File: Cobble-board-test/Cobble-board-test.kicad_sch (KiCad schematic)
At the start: 16 parts, among them J2 JST PH2.0 Battery, J3 Stemma PH, J4 Grove, Q1 SI2302DS, SW1 SW_Push, SW3 SW_VIBE, SW4 MSK22D27

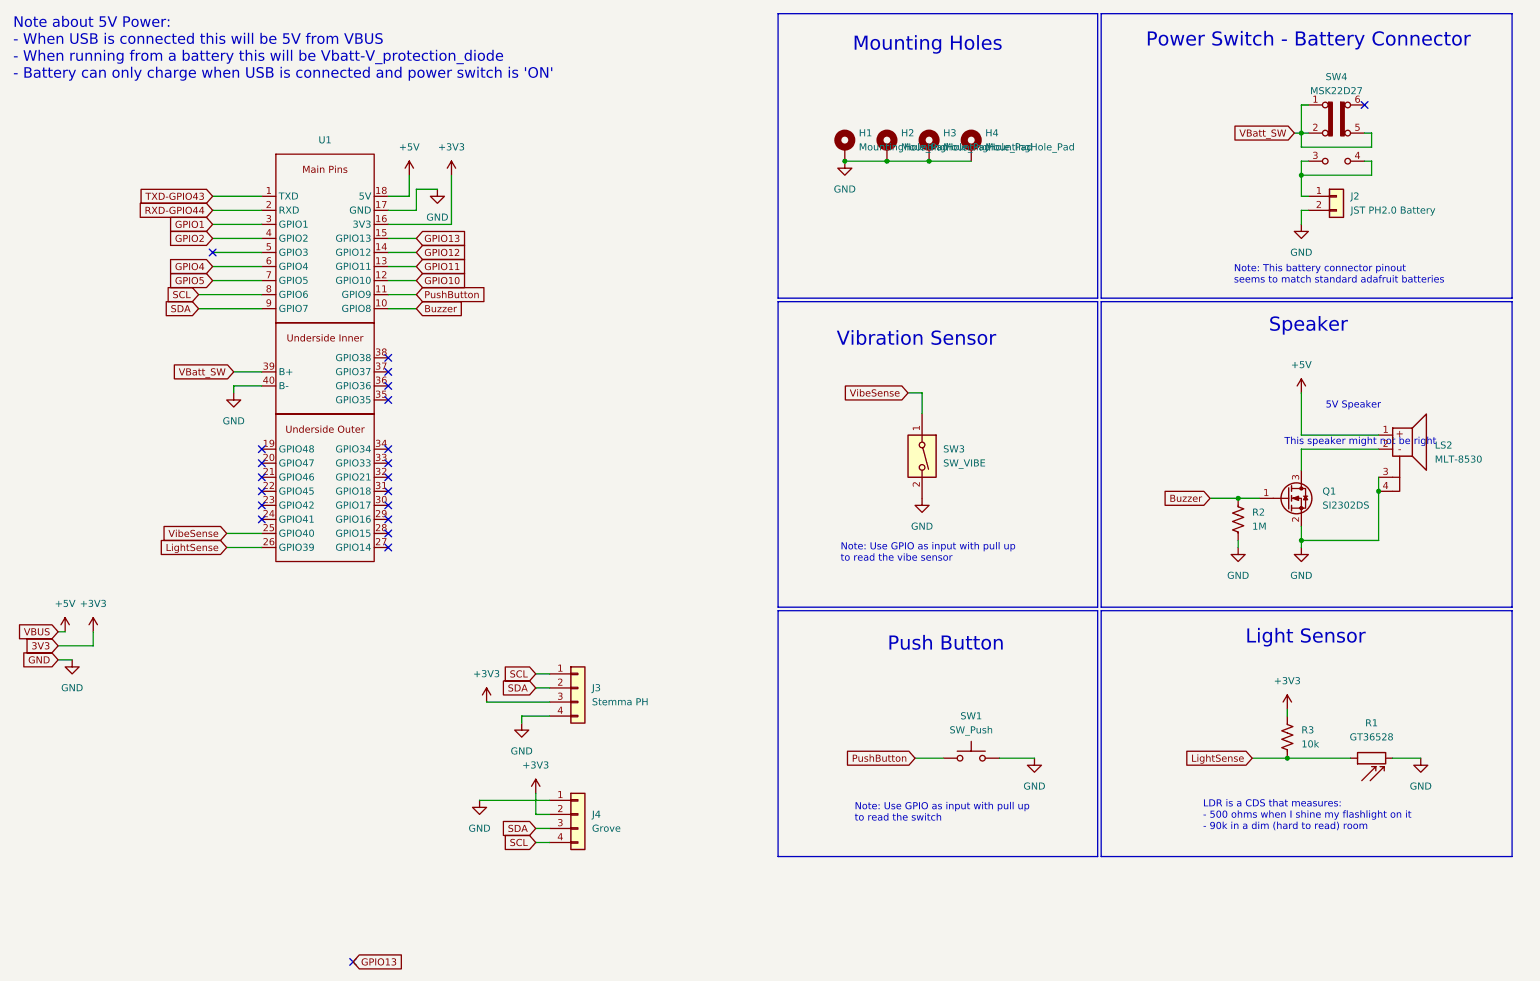
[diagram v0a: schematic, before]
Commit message: Cobbl-board-test is complete and tested
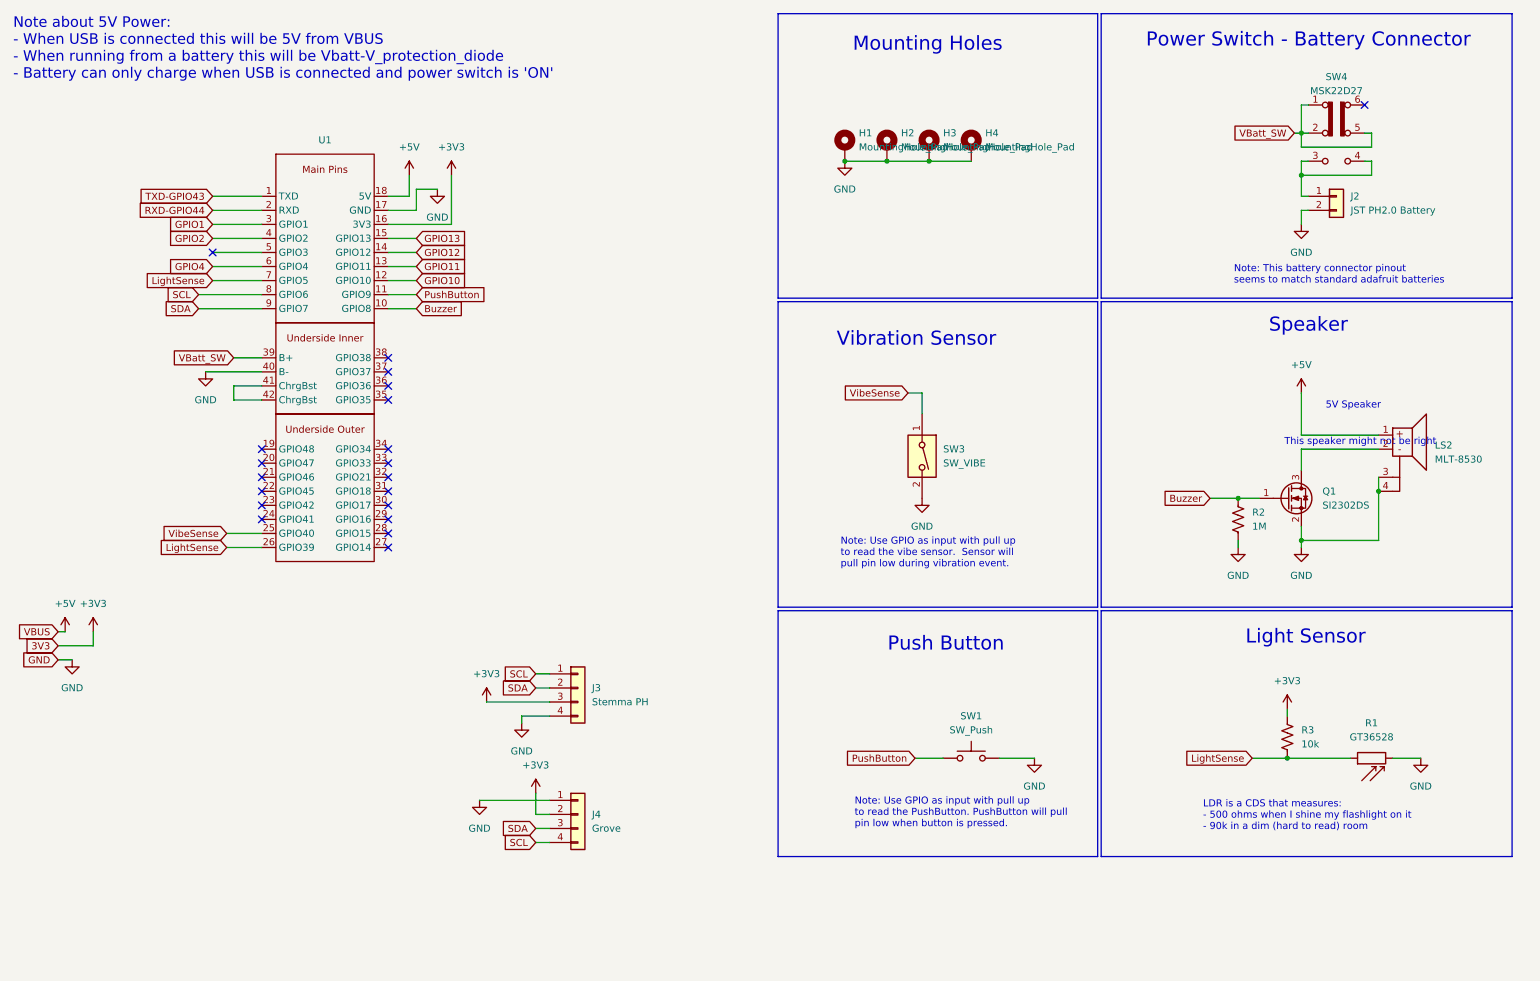
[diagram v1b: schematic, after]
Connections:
- net GPIO5 is gone; now on net LightSense: U1.7 (GPIO5)
- new net: U1.41 (ChrgBst), U1.42 (ChrgBst)
- no-connect marks 21 -> 20
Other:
- note added: "Note: Use GPIO as input with pull up to read the PushButton. PushButton will pull pin low when button is pressed."
- note added: "Note: Use GPIO as input with pull up to read the vibe sensor. Sensor will pull pin low during vibration event."
- note removed: "Note: Use GPIO as input with pull up to read the switch"
- note removed: "Note: Use GPIO as input with pull up to read the vibe sensor"
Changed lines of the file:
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@@
 		)
 	)
-	(text "Note: Use GPIO as input with pull up \nto read the switch"
+	(text "Note: Use GPIO as input with pull up \nto read the PushButton. PushButton will pull \npin low when button is pressed."
 		(exclude_from_sim no)
 		(at 165.608 157.226 0)
@@
 		)
 	)
-	(text "Note: Use GPIO as input with pull up \nto read the vibe sensor"
+	(text "Note: Use GPIO as input with pull up \nto read the vibe sensor.  Sensor will \npull pin low during vibration event."
 		(exclude_from_sim no)
 		(at 163.068 110.236 0)
@@
 	)
 	(no_connect
-		(at 74.93 184.15)
-	)
-	(no_connect
 		(at 81.28 74.93)
 	)
@@
 	(wire
 		(pts
-			(xy 53.34 77.47) (xy 58.42 77.47)
+			(xy 48.26 77.47) (xy 58.42 77.47)
 		)
 		(stroke
@@
 	(wire
 		(pts
+			(xy 53.34 74.93) (xy 58.42 74.93)
+		)
+		(stroke
+			(width 0)
+			(type default)
+		)
+	)
+	(wire
+		(pts
 			(xy 21.59 129.54) (xy 24.13 129.54)
 		)
@@
 	(wire
 		(pts
-			(xy 53.34 80.01) (xy 53.34 81.28)
+			(xy 53.34 80.01) (xy 53.34 82.55)
 		)
 		(stroke
@@
 	(wire
 		(pts
+			(xy 53.34 82.55) (xy 58.42 82.55)
+		)
+		(stroke
+			(width 0)
+			(type default)
+		)
+	)
+	(wire
+		(pts
 			(xy 97.79 154.94) (xy 110.49 154.94)
 		)
@@
 		)
 	)
-	(global_label "GPIO13"
+	(global_label "LightSense"
 		(shape input)
-		(at 74.93 184.15 0)
+		(at 49.53 60.96 180)
 		(fields_autoplaced yes)
 		(effects
@@
 				(size 1.27 1.27)
 			)
-			(justify left)
+			(justify right)
 		)
 		(property "Intersheetrefs" "${INTERSHEET_REFS}"
-			(at 84.8095 184.15 0)
+			(at 36.3244 60.96 0)
 			(hide yes)
 			(show_name no)
@@
 					(size 1.27 1.27)
 				)
-				(justify left)
+				(justify right)
 			)
 		)
@@
 	(global_label "VBatt_SW"
 		(shape input)
-		(at 53.34 77.47 180)
+		(at 53.34 74.93 180)
 		(fields_autoplaced yes)
 		(effects
@@
 		)
 		(property "Intersheetrefs" "${INTERSHEET_REFS}"
-			(at 41.7673 77.47 0)
+			(at 41.7673 74.93 0)
 			(hide yes)
 			(show_name no)
@@
 		)
 	)
-	(global_label "GPIO5"
-		(shape input)
-		(at 49.53 60.96 180)
-		(fields_autoplaced yes)
-		(effects
-			(font
-				(size 1.27 1.27)
-			)
-			(justify right)
-		)
-		(property "Intersheetrefs" "${INTERSHEET_REFS}"
-			(at 40.86 60.96 0)
-			(hide yes)
-			(show_name no)
-			(do_not_autoplace no)
-			(effects
-				(font
-					(size 1.27 1.27)
-				)
-				(justify right)
-			)
-		)
-	)
 	(global_label "SCL"
 		(shape input)
@@
 		(pin "16"
 		)
+		(pin "42"
+		)
+		(pin "41"
+		)
 		(instances
 			(project "Cobble-board-test"
@@
 	(symbol
 		(lib_id "power:GND")
-		(at 53.34 81.28 0)
+		(at 48.26 77.47 0)
 		(unit 1)
 		(body_style 1)
@@
 		(fields_autoplaced yes)
 		(property "Reference" "#PWR013"
-			(at 53.34 87.63 0)
+			(at 48.26 83.82 0)
 			(hide yes)
 			(show_name no)
@@
 		)
 		(property "Value" "GND"
-			(at 53.34 86.36 0)
+			(at 48.26 82.55 0)
 			(show_name no)
 			(do_not_autoplace no)
@@
 		)
 		(property "Footprint" ""
-			(at 53.34 81.28 0)
+			(at 48.26 77.47 0)
 			(hide yes)
 			(show_name no)
@@
 		)
 		(property "Datasheet" ""
-			(at 53.34 81.28 0)
+			(at 48.26 77.47 0)
 			(hide yes)
 			(show_name no)
@@
 		)
 		(property "Description" "Power symbol creates a global label with name \"GND\" , ground"
-			(at 53.34 81.28 0)
+			(at 48.26 77.47 0)
 			(hide yes)
 			(show_name no)

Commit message: Cobble board is rev 1 is ready for review
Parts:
- U1: footprint Cobble_Library:ESP32S3-supermini -> Cobble_Library:ESP32S3-supermini-v2
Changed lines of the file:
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@@
 			)
 		)
-		(property "Footprint" "Cobble_Library:ESP32S3-supermini"
+		(property "Footprint" "Cobble_Library:ESP32S3-supermini-v2"
 			(at 69.85 53.34 0)
 			(hide yes)
